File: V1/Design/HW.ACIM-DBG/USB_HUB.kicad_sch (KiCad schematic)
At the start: 59 parts, among them J1 USB C, Q2 MFET N, U1 LDO 3.3V, U2 USB HUB 2.0 4-CH, U4 USB PD, U5 eFuse, Y1 24MHz

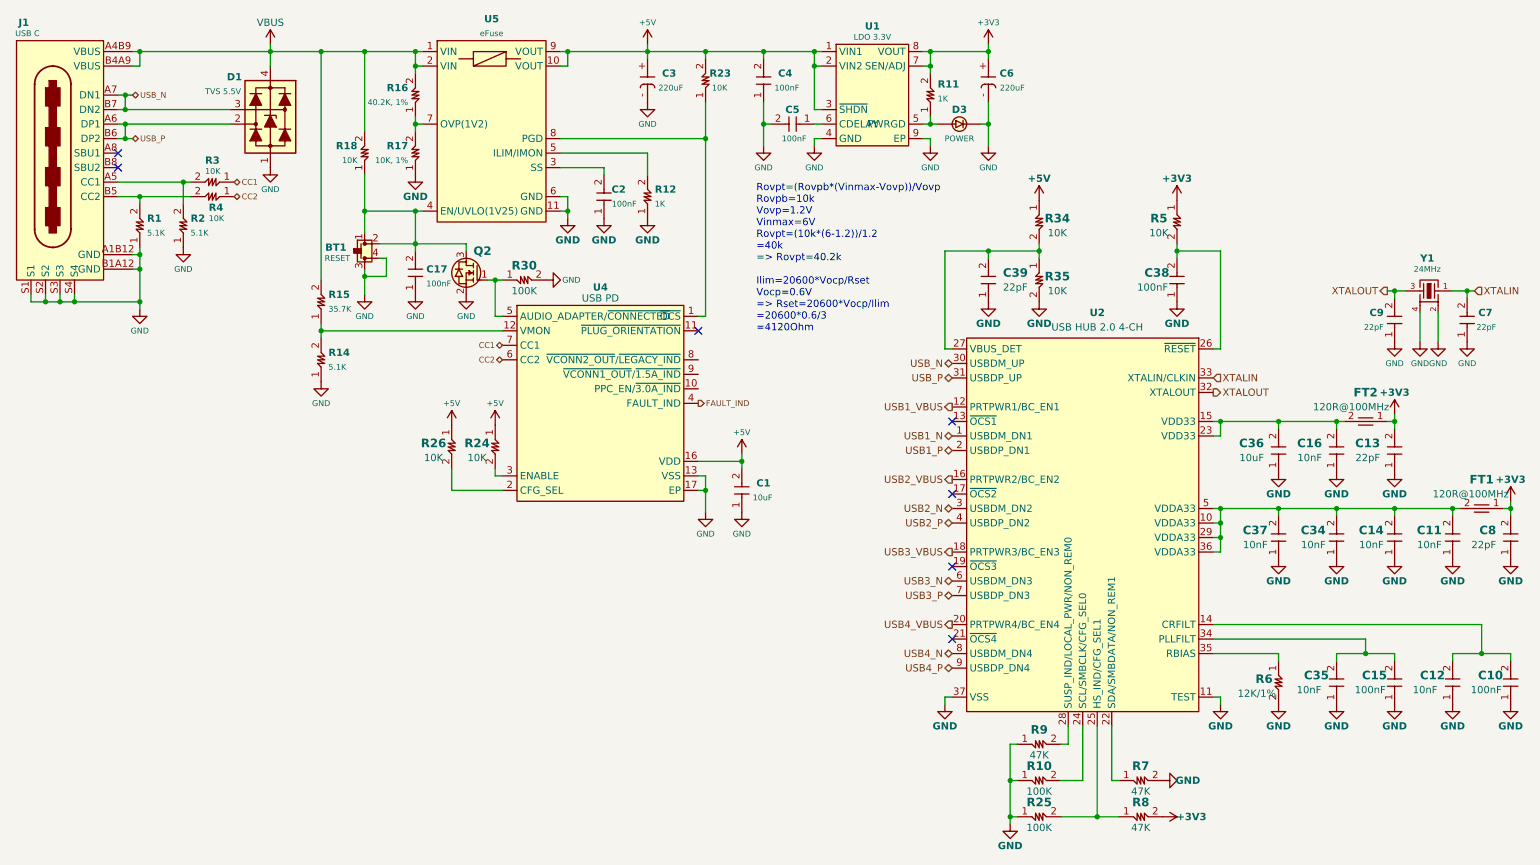
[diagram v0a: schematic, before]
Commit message: V1 layout update 8
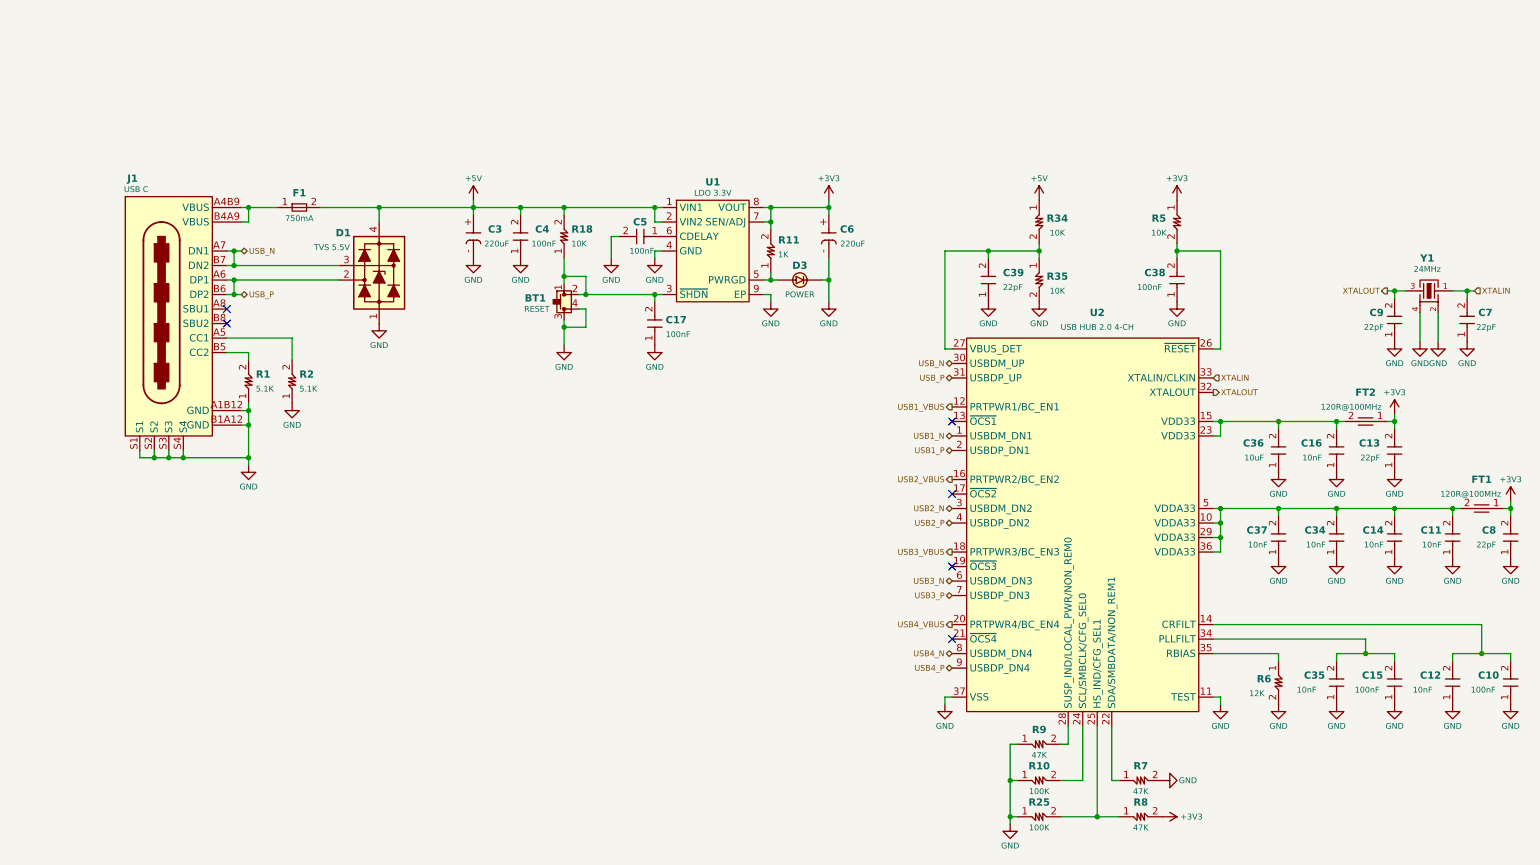
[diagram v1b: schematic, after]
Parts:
- removed C1: 10uF, SAMPI:CAP0603, symbol SAMPI:CERCAP
- removed C2: 100nF, SAMPI:CAP0603, symbol SAMPI:CERCAP
- removed Q2: MFET N, SAMPI:SOT23, symbol SAMPI:FET_N-CH
- removed R12: 1K, SAMPI:RES0603, symbol SAMPI:RES
- removed R14: 5.1K, SAMPI:RES0603, symbol SAMPI:RES
- removed R15: 35.7K, SAMPI:RES0603, symbol SAMPI:RES
- removed R16: 40.2K, 1%, SAMPI:RES0603, symbol SAMPI:RES
- removed R17: 10K, 1%, SAMPI:RES0603, symbol SAMPI:RES
- removed R23, R24, R26, R3, R4: 10K, SAMPI:RES0603, symbol SAMPI:RES
- removed R30: 100K, SAMPI:RES0603, symbol SAMPI:RES
- removed U4: USB PD, SAMPI:QFN16, symbol Liem:UTC2000
- removed U5: eFuse, SAMPI:DFN10-EP-3x3, symbol SAMPI:eFUSE
- added F1: 750mA, Liem:FUSE1812, symbol Liem:FUSE
- BT1: MFT CUI -> SCHUR; MNP TS02-66-170-BK-160-SCR-D -> 1301.9304
- C10, C15, C17, C38, C4, C5: MFT Samsung -> YAGE; MNP CL10B104KB8NNNC -> CC0603ZRY5V9BB104
- C11, C12, C14, C16, C34, C35, C37: MFT YAGEO -> MRTN; MNP CC0603KRX7R9BB103 -> GRM188R71H103KA01D
- C13, C39, C7, C8, C9: MFT Walsin -> YAGE; MNP 0603N220J500CT -> CC0603JRNPO9BN220
- C3, C6: MFT Vishay Sprague -> NCHC; MNP 293D227X96R3C2TE3 -> F930J227KBA
- C36: MFT Samsung -> TAIY; MNP CL10A106MQ8NNNC -> EMK107BBJ106MA-T
- D3: MFT Würth Elektronik -> ROHM; MNP 151031VS06000 -> SML-D12M8WT86
- FT1, FT2: MFT Pulse -> TDK; MNP PE-0603PFB121ST -> MPZ1608S121ATAH0
- R1, R2: MFT YAGEO -> YAGE
- R10, R25: MFT YAGEO -> NIC; MNP RC0603FR-07100KL -> NRC06F1003TRF
- R11: MFT YAGEO -> ROHM; MNP RC0603FR-071KL -> MCR03PZPZFX1001
- R6: value 12K/1% -> 12K
- Y1: footprint SAMPI:CDFN3225-4LD-PL-1 -> SAMPI:CDFN2520-ABM10; MFT Abracon LLC -> CTSF; MNP ABM8AIG-24.000MHZ-12-2Z-T3 -> 425F35B024M0000
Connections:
- net +5V: now also D1.4 (VCC), R18.2, F1.2; no longer U1.3 (~{SHDN})
- net at BT1.1, BT1.2, C17.2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: now also U1.3 (~{SHDN})
- net VBUS: no longer names the net of J1.A4B9 (VBUS), J1.B4A9 (VBUS)
- net VBUS: now also F1.1; no longer D1.4 (VCC), R18.2
- no-connect marks 7 -> 6
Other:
- note removed: "Rovpt=(Rovpb*(Vinmax-Vovp))/Vovp Rovpb=10k Vovp=1.2V Vinmax=6V Rovpt=(10k*(6-1.2))/1.2 =40k => Rovpt=40.2k Ilim=20600*Vocp/Rset Vocp=0.6V => Rset=20600*Vocp/Ilim =20600*0.6/3 =4120Ohm"
- moved on the sheet: BT1, C17, C3, C4, C5, C6, D1, D3, J1, R1, R11, R18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
